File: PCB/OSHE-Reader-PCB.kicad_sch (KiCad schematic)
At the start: 2 parts

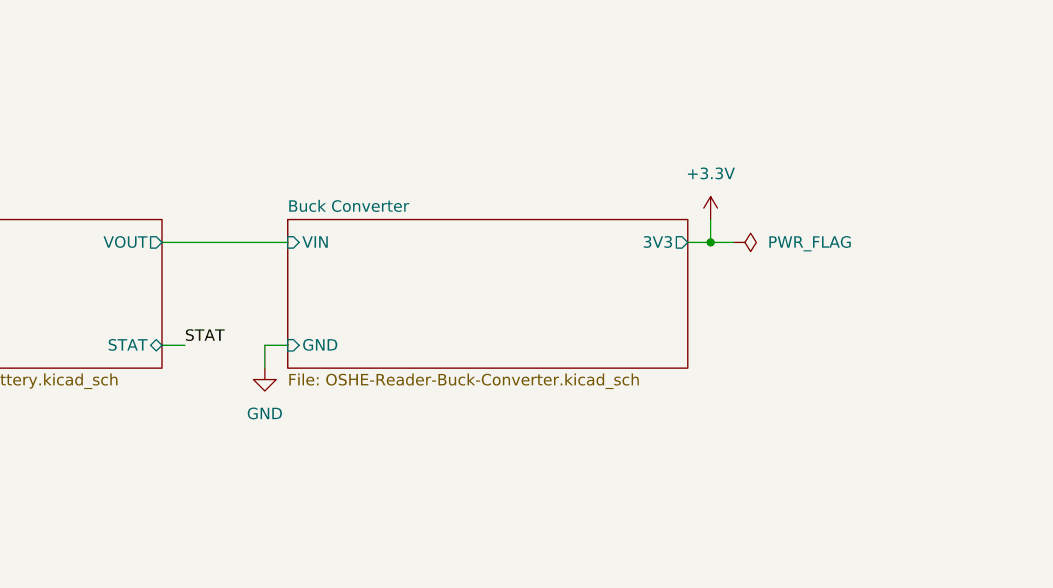
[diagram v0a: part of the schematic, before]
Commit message: started work adding hierarchical power pins to mcu and sd card sheets
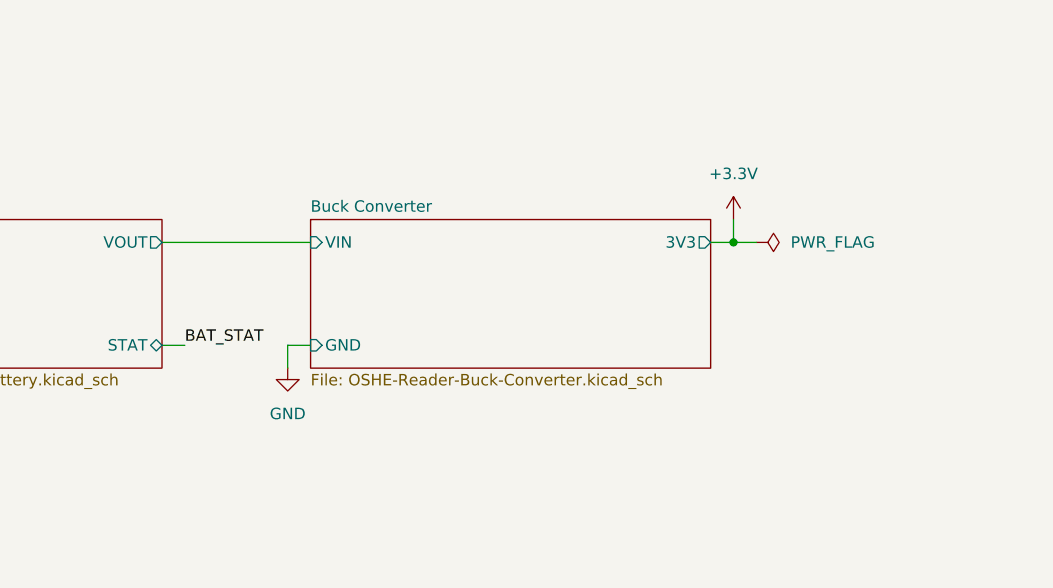
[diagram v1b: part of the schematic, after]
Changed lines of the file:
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@@
 	)
 	(junction
-		(at 201.93 125.73)
+		(at 204.47 125.73)
 		(diameter 0)
 		(color 0 0 0 0)
@@
 	(wire
 		(pts
-			(xy 201.93 123.19) (xy 201.93 125.73)
+			(xy 204.47 123.19) (xy 204.47 125.73)
+		)
+		(stroke
+			(width 0)
+			(type default)
+		)
+	)
+	(wire
+		(pts
+			(xy 204.47 125.73) (xy 207.01 125.73)
+		)
+		(stroke
+			(width 0)
+			(type default)
+		)
+	)
+	(wire
+		(pts
+			(xy 140.97 125.73) (xy 157.48 125.73)
+		)
+		(stroke
+			(width 0)
+			(type default)
+		)
+	)
+	(wire
+		(pts
+			(xy 87.63 166.37) (xy 87.63 162.56)
+		)
+		(stroke
+			(width 0)
+			(type default)
+		)
+	)
+	(wire
+		(pts
+			(xy 90.17 166.37) (xy 90.17 168.91)
+		)
+		(stroke
+			(width 0)
+			(type default)
+		)
+	)
+	(wire
+		(pts
+			(xy 87.63 154.94) (xy 87.63 129.54)
+		)
+		(stroke
+			(width 0)
+			(type default)
+		)
+	)
+	(wire
+		(pts
+			(xy 30.48 137.16) (xy 33.02 137.16)
+		)
+		(stroke
+			(width 0)
+			(type default)
+		)
+	)
+	(wire
+		(pts
+			(xy 30.48 137.16) (xy 30.48 139.7)
+		)
+		(stroke
+			(width 0)
+			(type default)
+		)
+	)
+	(wire
+		(pts
+			(xy 81.28 125.73) (xy 104.14 125.73)
+		)
+		(stroke
+			(width 0)
+			(type default)
+		)
+	)
+	(wire
+		(pts
+			(xy 92.71 133.35) (xy 104.14 133.35)
+		)
+		(stroke
+			(width 0)
+			(type default)
+		)
+	)
+	(wire
+		(pts
+			(xy 90.17 166.37) (xy 92.71 166.37)
 		)
 		(stroke
@@
 	(wire
 		(pts
-			(xy 140.97 125.73) (xy 154.94 125.73)
-		)
-		(stroke
-			(width 0)
-			(type default)
-		)
-	)
-	(wire
-		(pts
-			(xy 87.63 166.37) (xy 87.63 162.56)
-		)
-		(stroke
-			(width 0)
-			(type default)
-		)
-	)
-	(wire
-		(pts
-			(xy 90.17 166.37) (xy 90.17 168.91)
-		)
-		(stroke
-			(width 0)
-			(type default)
-		)
-	)
-	(wire
-		(pts
-			(xy 87.63 154.94) (xy 87.63 129.54)
-		)
-		(stroke
-			(width 0)
-			(type default)
-		)
-	)
-	(wire
-		(pts
-			(xy 30.48 137.16) (xy 33.02 137.16)
-		)
-		(stroke
-			(width 0)
-			(type default)
-		)
-	)
-	(wire
-		(pts
-			(xy 30.48 137.16) (xy 30.48 139.7)
-		)
-		(stroke
-			(width 0)
-			(type default)
-		)
-	)
-	(wire
-		(pts
-			(xy 81.28 125.73) (xy 104.14 125.73)
-		)
-		(stroke
-			(width 0)
-			(type default)
-		)
-	)
-	(wire
-		(pts
-			(xy 92.71 133.35) (xy 104.14 133.35)
-		)
-		(stroke
-			(width 0)
-			(type default)
-		)
-	)
-	(wire
-		(pts
-			(xy 90.17 166.37) (xy 92.71 166.37)
-		)
-		(stroke
-			(width 0)
-			(type default)
-		)
-	)
-	(wire
-		(pts
-			(xy 199.39 125.73) (xy 201.93 125.73)
-		)
-		(stroke
-			(width 0)
-			(type default)
-		)
-	)
-	(wire
-		(pts
 			(xy 92.71 153.67) (xy 92.71 133.35)
 		)
@@
 	(wire
 		(pts
-			(xy 152.4 137.16) (xy 152.4 139.7)
+			(xy 154.94 137.16) (xy 154.94 139.7)
 		)
 		(stroke
@@
 	(wire
 		(pts
-			(xy 152.4 137.16) (xy 154.94 137.16)
-		)
-		(stroke
-			(width 0)
-			(type default)
-		)
-	)
-	(label "STAT"
+			(xy 154.94 137.16) (xy 157.48 137.16)
+		)
+		(stroke
+			(width 0)
+			(type default)
+		)
+	)
+	(label "BAT_STAT"
 		(at 143.51 137.16 0)
 		(effects
@@
 	(symbol
 		(lib_id "power:GND")
-		(at 152.4 139.7 0)
+		(at 154.94 139.7 0)
 		(unit 1)
 		(exclude_from_sim no)
@@
 		(fields_autoplaced yes)
 		(property "Reference" "#PWR03"
-			(at 152.4 146.05 0)
+			(at 154.94 146.05 0)
 			(effects
 				(font
@@
 		)
 		(property "Value" "GND"
-			(at 152.4 144.78 0)
+			(at 154.94 144.78 0)
 			(effects
 				(font
@@
 		)
 		(property "Footprint" ""
-			(at 152.4 139.7 0)
+			(at 154.94 139.7 0)
 			(effects
 				(font
@@
 		)
 		(property "Datasheet" ""
-			(at 152.4 139.7 0)
+			(at 154.94 139.7 0)
 			(effects
 				(font
@@
 		)
 		(property "Description" "Power symbol creates a global label with name \"GND\" , ground"
-			(at 152.4 139.7 0)
+			(at 154.94 139.7 0)
 			(effects
 				(font
@@
 	(symbol
 		(lib_id "power:PWR_FLAG")
-		(at 204.47 125.73 270)
+		(at 207.01 125.73 270)
 		(unit 1)
 		(exclude_from_sim no)
@@
 		(fields_autoplaced yes)
 		(property "Reference" "#FLG02"
-			(at 206.375 125.73 0)
+			(at 208.915 125.73 0)
 			(effects
 				(font
@@
 		)
 		(property "Value" "PWR_FLAG"
-			(at 208.28 125.7299 90)
+			(at 210.82 125.7299 90)
 			(effects
 				(font
@@
 		)
 		(property "Footprint" ""
-			(at 204.47 125.73 0)
+			(at 207.01 125.73 0)
 			(effects
 				(font
@@
 		)
 		(property "Datasheet" "~"
-			(at 204.47 125.73 0)
+			(at 207.01 125.73 0)
 			(effects
 				(font
@@
 		)
 		(property "Description" "Special symbol for telling ERC where power comes from"
-			(at 204.47 125.73 0)
+			(at 207.01 125.73 0)
 			(effects
 				(font
@@
 	(symbol
 		(lib_id "power:+3.3V")
-		(at 201.93 123.19 0)
+		(at 204.47 123.19 0)
 		(unit 1)
 		(exclude_from_sim no)
@@
 		(fields_autoplaced yes)
 		(property "Reference" "#PWR04"
-			(at 201.93 127 0)
+			(at 204.47 127 0)
 			(effects
 				(font
@@
 		)
 		(property "Value" "+3.3V"
-			(at 201.93 118.11 0)
+			(at 204.47 118.11 0)
 			(effects
 				(font
@@
 		)
 		(property "Footprint" ""
-			(at 201.93 123.19 0)
+			(at 204.47 123.19 0)
 			(effects
 				(font
@@
 		)
 		(property "Datasheet" ""
-			(at 201.93 123.19 0)
+			(at 204.47 123.19 0)
 			(effects
 				(font
@@
 		)
 		(property "Description" "Power symbol creates a global label with name \"+3.3V\""
-			(at 201.93 123.19 0)
+			(at 204.47 123.19 0)
 			(effects
 				(font
@@
 	)
 	(sheet
-		(at 154.94 123.19)
+		(at 157.48 123.19)
 		(size 44.45 16.51)
 		(exclude_from_sim no)
@@
 		)
 		(property "Sheetname" "Buck Converter"
-			(at 154.94 122.4784 0)
+			(at 157.48 122.4784 0)
 			(effects
 				(font
@@
 		)
 		(property "Sheetfile" "OSHE-Reader-Buck-Converter.kicad_sch"
-			(at 154.94 140.2846 0)
+			(at 157.48 140.2846 0)
 			(effects
 				(font
@@
 		)
 		(pin "GND" input
-			(at 154.94 137.16 180)
+			(at 157.48 137.16 180)
 			(effects
 				(font
@@
 		)
 		(pin "VIN" input
-			(at 154.94 125.73 180)
+			(at 157.48 125.73 180)
 			(effects
 				(font
@@
 		)
 		(pin "3V3" output
-			(at 199.39 125.73 0)
-			(effects
-				(font
+			(at 201.93 125.73 0)
+			(effects
+				(font
